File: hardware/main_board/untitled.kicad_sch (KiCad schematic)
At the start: 37 parts, among them IC4 TPS2121RUXT, IC5 TP5000-QFN16, J3 Solar panel, J4 USB4105-GF-A-060, J5 Battary over BMS, U4 TPS631000DRLR

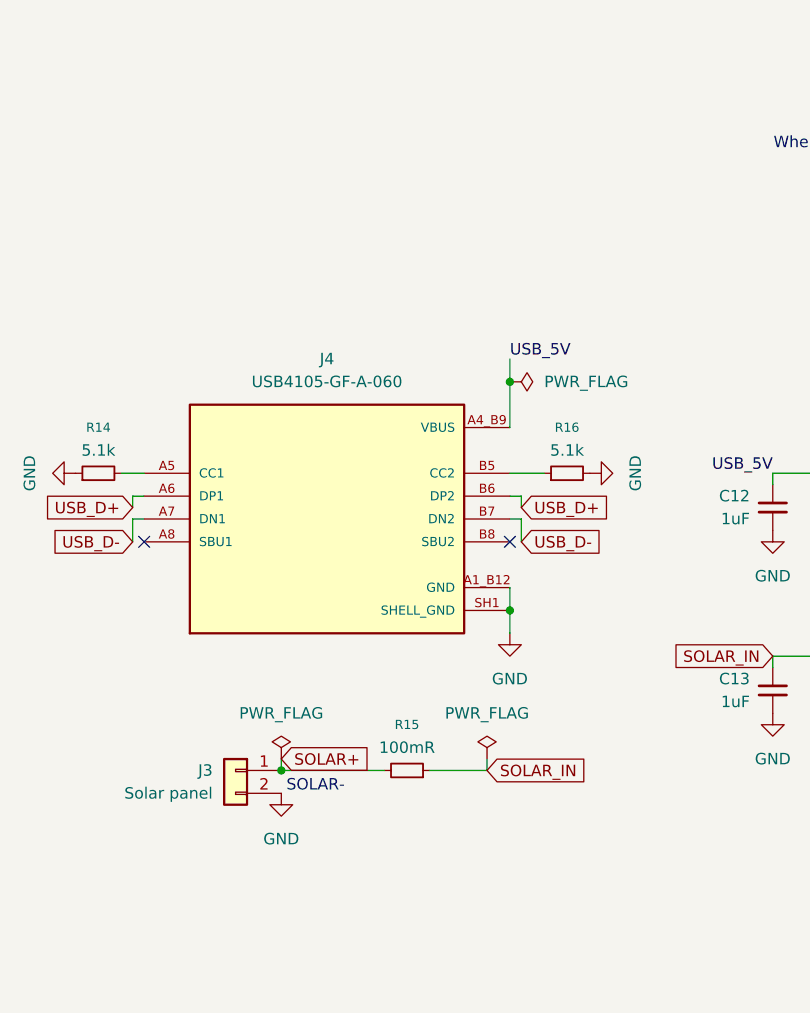
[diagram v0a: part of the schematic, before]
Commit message: hw start board
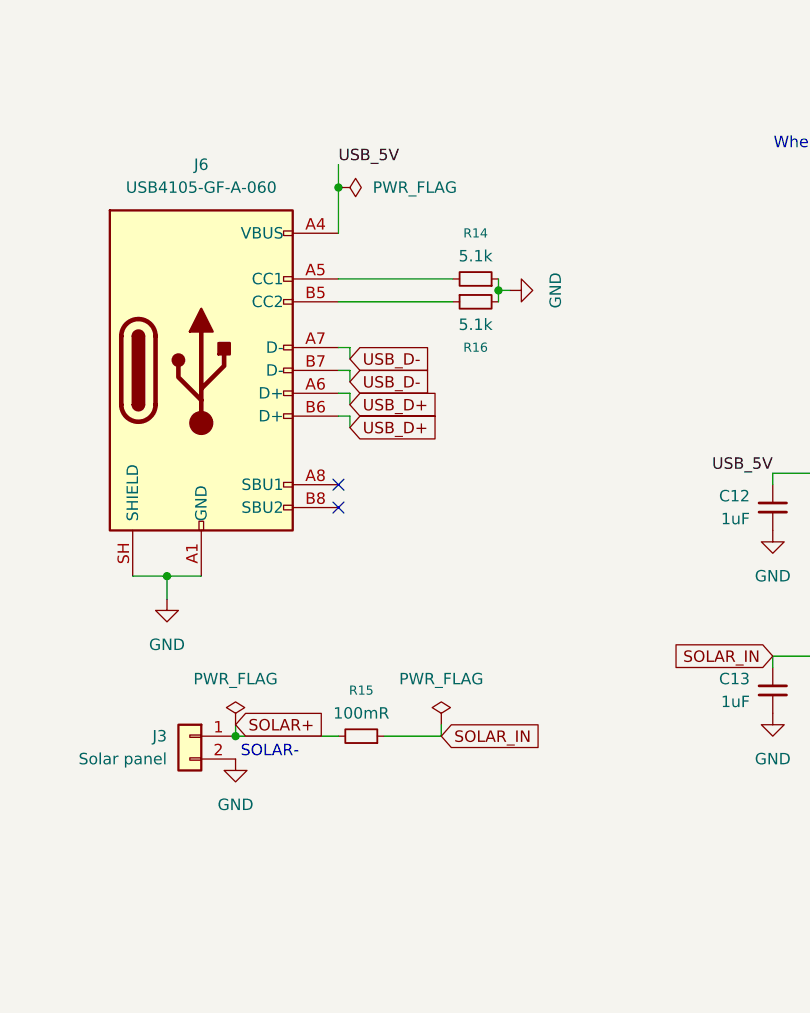
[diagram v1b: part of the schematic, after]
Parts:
- removed J4: USB4105-GF-A-060, USB4105-GF-A-060:GCT_USB4105-GF-A-060, symbol USB4105-GF-A-060:USB4105-GF-A-060
- added J6: USB4105-GF-A-060, Connector_USB:USB_C_Receptacle_GCT_USB4105-xx-A_16P_TopMnt_Horizontal, symbol Connector:USB_C_Receptacle_USB2.0_16P
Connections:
- net GND: now also J6.A1 (GND), J6.A12 (GND), J6.B1 (GND), J6.B12 (GND), J6.SH (SHIELD)
- net USB_5V: now also J6.A4 (VBUS), J6.A9 (VBUS), J6.B4 (VBUS), J6.B9 (VBUS)
- net USB_D+: now also J6.A6 (D+), J6.B6 (D+)
- net USB_D-: now also J6.A7 (D-), J6.B7 (D-)
- net at R14.2: now also J6.A5 (CC1)
- net at R16.1: now also J6.B5 (CC2)
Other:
- moved on the sheet: J3, R15
